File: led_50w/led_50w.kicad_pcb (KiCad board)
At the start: 2 copper layers, 120 x 80 mm, 51 parts

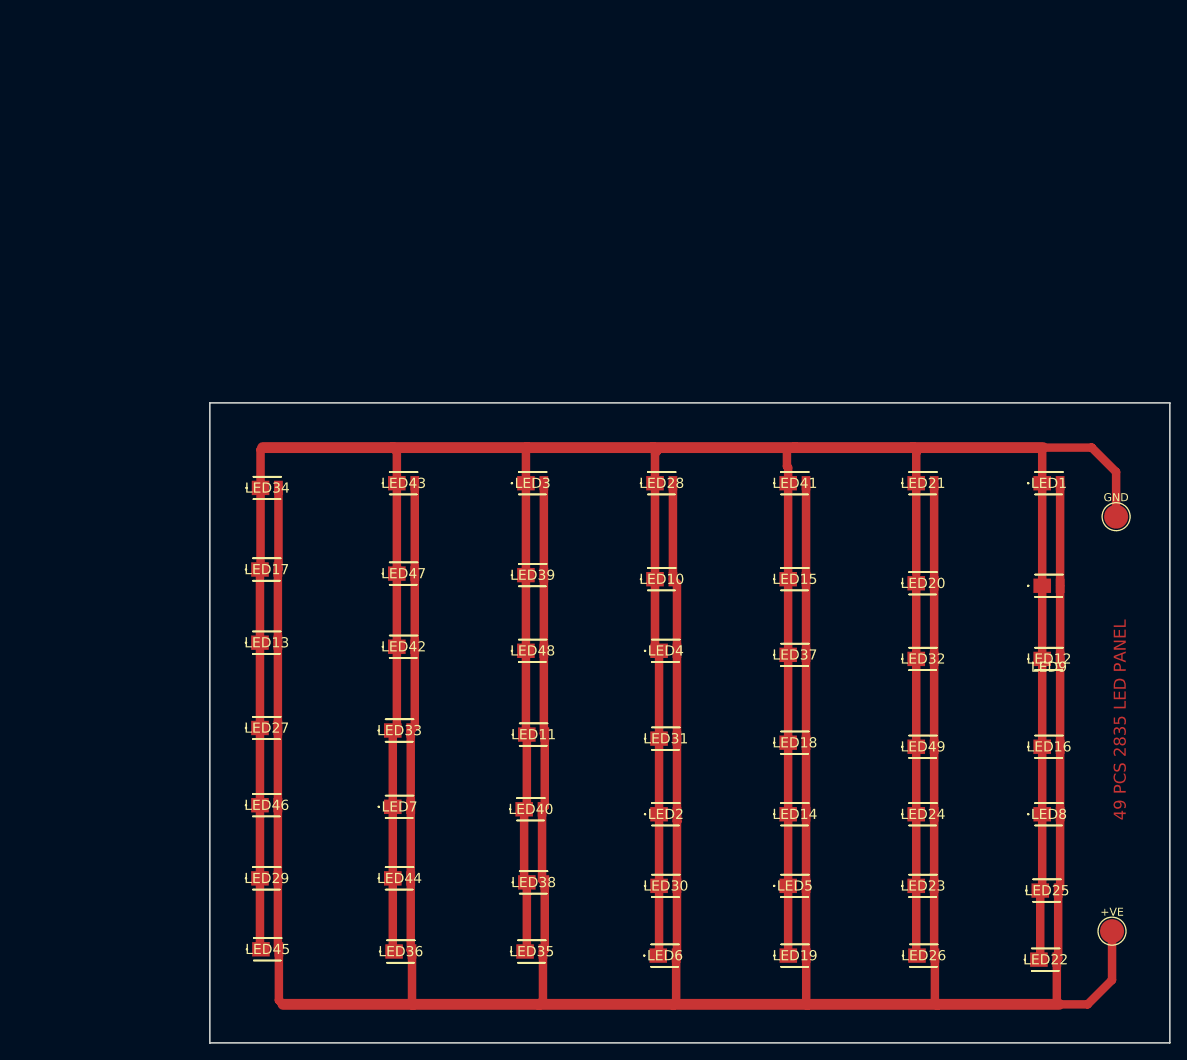
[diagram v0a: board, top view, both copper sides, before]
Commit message: RECTIFIED CONNECTION
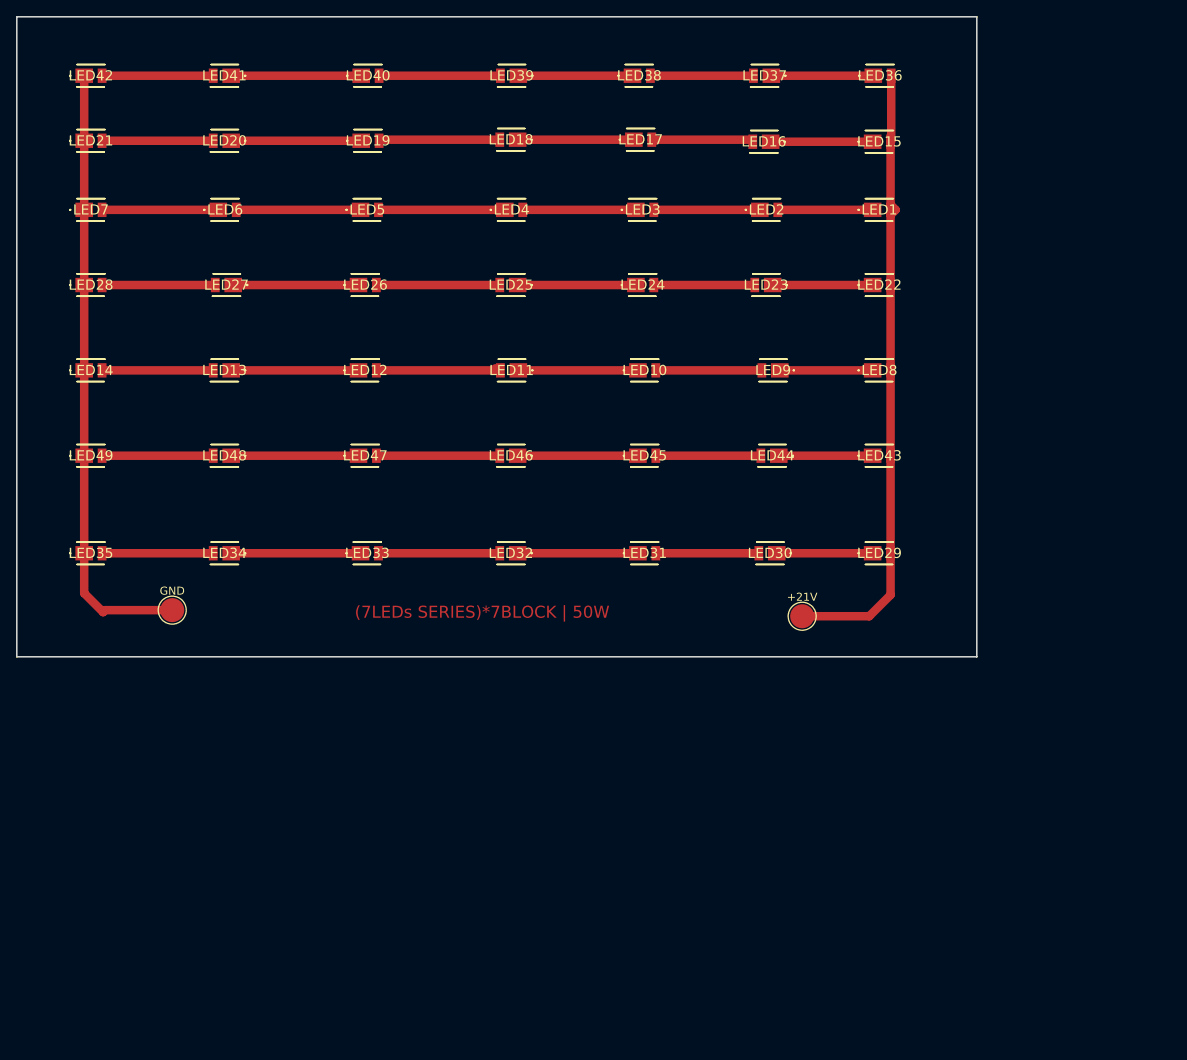
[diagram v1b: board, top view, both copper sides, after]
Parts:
- removed +VE: TestPoint, TestPoint:TestPoint_Pad_D3.0mm
- added +21V: TestPoint, TestPoint:TestPoint_Pad_D3.0mm, F.Cu at (145.7, 89.7)
- moved LED36 124.8 mm to (154.6, 22.1)
- moved GND 118.6 mm to (66.9, 88.9)
- moved LED19 115.0 mm to (90.5, 30.2)
- moved LED21 112.5 mm to (55.9, 30.2)
- moved LED49 110.2 mm to (55.9, 69.6)
- moved LED26 109.1 mm to (90.2, 48.3)
- moved LED6 108.2 mm to (72.7, 38.9)
- moved LED14 104.0 mm to (55.9, 58.9)
- moved LED20 101.9 mm to (74.3, 30.2), turned to 180 degrees
- moved LED38 101.7 mm to (124.5, 22.1)
- moved LED5 100.0 mm to (90.5, 38.9)
- moved LED25 100.0 mm to (110.1, 48.3), turned to 180 degrees
- moved LED40 93.9 mm to (90.5, 22.1)
- moved LED12 92.8 mm to (90.2, 58.9)
- moved LED22 86.9 mm to (154.5, 48.3)
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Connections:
- LED1 pad 1: GND -> Net-(LED1-Pad1)
- LED10 pad 1: GND -> Net-(LED10-Pad1)
- LED10 pad 2: +24V -> Net-(LED10-Pad2)
- LED11 pad 1: GND -> Net-(LED10-Pad1)
- LED11 pad 2: +24V -> Net-(LED11-Pad2)
- LED12 pad 1: GND -> Net-(LED12-Pad1)
- LED12 pad 2: +24V -> Net-(LED11-Pad2)
- LED13 pad 1: GND -> Net-(LED12-Pad1)
- LED13 pad 2: +24V -> Net-(LED13-Pad2)
- LED14 pad 2: +24V -> Net-(LED13-Pad2)
- LED15 pad 1: GND -> Net-(LED15-Pad1)
- LED16 pad 1: GND -> Net-(LED15-Pad1)
- LED16 pad 2: +24V -> Net-(LED16-Pad2)
- LED17 pad 1: GND -> Net-(LED17-Pad1)
- LED17 pad 2: +24V -> Net-(LED16-Pad2)
- LED18 pad 1: GND -> Net-(LED17-Pad1)
- LED18 pad 2: +24V -> Net-(LED18-Pad2)
- LED19 pad 1: GND -> Net-(LED19-Pad1)
- LED19 pad 2: +24V -> Net-(LED18-Pad2)
- LED2 pad 1: GND -> Net-(LED2-Pad1)
- LED2 pad 2: +24V -> Net-(LED1-Pad1)
- LED20 pad 1: GND -> Net-(LED19-Pad1)
- LED20 pad 2: +24V -> Net-(LED20-Pad2)
- LED21 pad 2: +24V -> Net-(LED20-Pad2)
- LED22 pad 1: GND -> Net-(LED22-Pad1)
- LED23 pad 1: GND -> Net-(LED22-Pad1)
- LED23 pad 2: +24V -> Net-(LED23-Pad2)
- LED24 pad 1: GND -> Net-(LED24-Pad1)
- LED24 pad 2: +24V -> Net-(LED23-Pad2)
- LED25 pad 1: GND -> Net-(LED24-Pad1)
- LED25 pad 2: +24V -> Net-(LED25-Pad2)
- LED26 pad 1: GND -> Net-(LED26-Pad1)
- LED26 pad 2: +24V -> Net-(LED25-Pad2)
- LED27 pad 1: GND -> Net-(LED26-Pad1)
- LED27 pad 2: +24V -> Net-(LED27-Pad2)
- LED28 pad 2: +24V -> Net-(LED27-Pad2)
- LED29 pad 1: GND -> Net-(LED29-Pad1)
- LED3 pad 1: GND -> Net-(LED3-Pad1)
- LED3 pad 2: +24V -> Net-(LED2-Pad1)
- LED30 pad 1: GND -> Net-(LED29-Pad1)
- LED30 pad 2: +24V -> Net-(LED30-Pad2)
- LED31 pad 1: GND -> Net-(LED31-Pad1)
- LED31 pad 2: +24V -> Net-(LED30-Pad2)
- LED32 pad 1: GND -> Net-(LED31-Pad1)
- LED32 pad 2: +24V -> Net-(LED32-Pad2)
- LED33 pad 1: GND -> Net-(LED33-Pad1)
- LED33 pad 2: +24V -> Net-(LED32-Pad2)
- LED34 pad 1: GND -> Net-(LED33-Pad1)
- LED34 pad 2: +24V -> Net-(LED34-Pad2)
- LED35 pad 2: +24V -> Net-(LED34-Pad2)
- LED36 pad 1: GND -> Net-(LED36-Pad1)
- LED37 pad 1: GND -> Net-(LED36-Pad1)
- LED37 pad 2: +24V -> Net-(LED37-Pad2)
- LED38 pad 1: GND -> Net-(LED38-Pad1)
- LED38 pad 2: +24V -> Net-(LED37-Pad2)
- LED39 pad 1: GND -> Net-(LED38-Pad1)
- LED39 pad 2: +24V -> Net-(LED39-Pad2)
- LED4 pad 1: GND -> Net-(LED4-Pad1)
- LED4 pad 2: +24V -> Net-(LED3-Pad1)
- LED40 pad 1: GND -> Net-(LED40-Pad1)
- LED40 pad 2: +24V -> Net-(LED39-Pad2)
- LED41 pad 1: GND -> Net-(LED40-Pad1)
- LED41 pad 2: +24V -> Net-(LED41-Pad2)
- LED42 pad 2: +24V -> Net-(LED41-Pad2)
- LED43 pad 1: GND -> Net-(LED43-Pad1)
- LED44 pad 1: GND -> Net-(LED43-Pad1)
- LED44 pad 2: +24V -> Net-(LED44-Pad2)
- LED45 pad 1: GND -> Net-(LED45-Pad1)
- LED45 pad 2: +24V -> Net-(LED44-Pad2)
- LED46 pad 1: GND -> Net-(LED45-Pad1)
- LED46 pad 2: +24V -> Net-(LED46-Pad2)
- LED47 pad 1: GND -> Net-(LED47-Pad1)
- LED47 pad 2: +24V -> Net-(LED46-Pad2)
- LED48 pad 1: GND -> Net-(LED47-Pad1)
- LED48 pad 2: +24V -> Net-(LED48-Pad2)
- LED49 pad 2: +24V -> Net-(LED48-Pad2)
- LED5 pad 1: GND -> Net-(LED5-Pad1)
- LED5 pad 2: +24V -> Net-(LED4-Pad1)
- LED6 pad 1: GND -> Net-(LED6-Pad1)
- LED6 pad 2: +24V -> Net-(LED5-Pad1)
- LED7 pad 2: +24V -> Net-(LED6-Pad1)
- LED8 pad 1: GND -> Net-(LED8-Pad1)
- LED9 pad 1: GND -> Net-(LED8-Pad1)
- LED9 pad 2: +24V -> Net-(LED10-Pad2)
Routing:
- net +24V: track 568.6 -> 77.6 mm
- net GND: track 558.9 -> 76.8 mm
- net Net-(LED40-Pad1): track 0.00 -> 16.3 mm
- net Net-(LED19-Pad1): track 0.00 -> 16.3 mm
- net Net-(LED33-Pad1): track 0.00 -> 16.2 mm
- net Net-(LED47-Pad1): track 0.00 -> 15.9 mm
- net Net-(LED12-Pad1): track 0.00 -> 15.9 mm
- net Net-(LED4-Pad1): track 0.00 -> 15.8 mm
- net Net-(LED26-Pad1): track 0.00 -> 15.7 mm
- net Net-(LED5-Pad1): track 0.00 -> 15.5 mm
- net Net-(LED46-Pad2): track 0.00 -> 15.4 mm
- net Net-(LED25-Pad2): track 0.00 -> 15.4 mm
- net Net-(LED39-Pad2): track 0.00 -> 15.2 mm
- net Net-(LED32-Pad2): track 0.00 -> 15.2 mm
- net Net-(LED18-Pad2): track 0.00 -> 15.1 mm
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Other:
- board text added: "(7LEDs SERIES)*7BLOCK | 50W"
- board text removed: "49 PCS 2835 LED PANEL"
